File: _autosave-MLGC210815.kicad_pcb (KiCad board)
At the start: 2 copper layers, 95 x 24 mm, 110 parts, among them J1 PinHeader_01x06_Male, J2 USB-B-04PFHTW, J3 PinHeader_01x01_Male, J4 PinHeader_01x01_Male, J5 PinHeader_01x02_Male, Q1 P-MOSFET_SI2315BDS-T1-E3, Q2 NPN_BC817, Q3 NPN_BC817, Q4 P-MOSFET_SI2315BDS-T1-E3, SW1 Switch-Tact_OMRON-B3F-3100, SW2 Switch-Tact_OMRON-B3F-3100, SW3 Switch-Tact_OMRON-B3F-3100, U1 PIC32MX170F256B-ISS, U2 OPA_MCP6V36T-E_OT, U3 LDO_MCP1700T-3302E_TT, U4 SENSOR_BMA250E, U5 INTERFACE_FT230XS, U6 BATTERY_MCP73833-FCI_UN, U7 DISPLAY_REX012832FWPP3N01, Y1 Crystal_SMD3225_12MHz

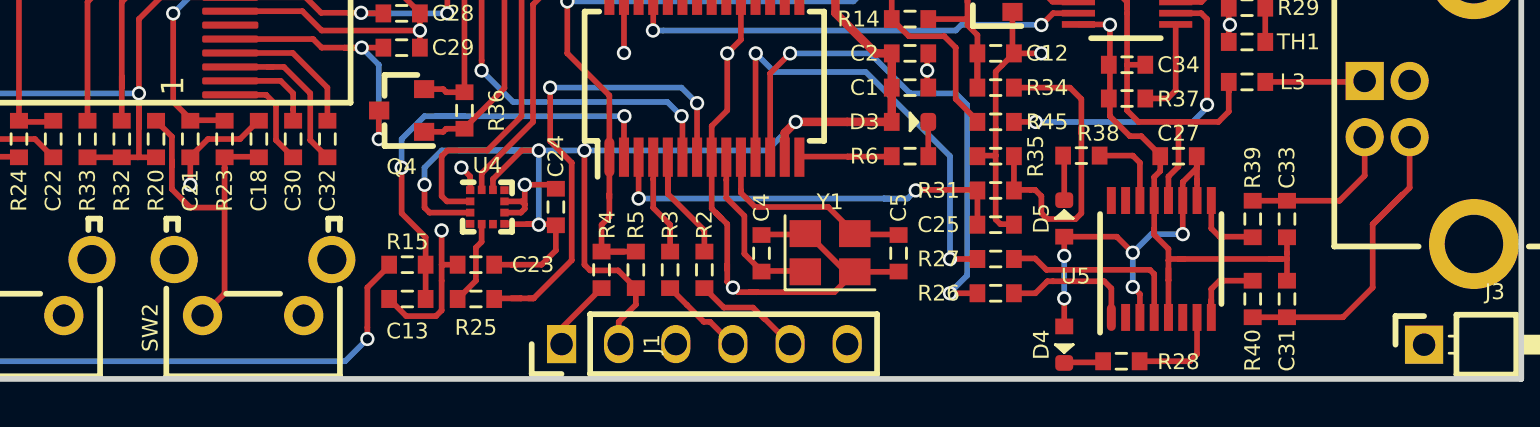
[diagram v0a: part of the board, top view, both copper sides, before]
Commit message: update
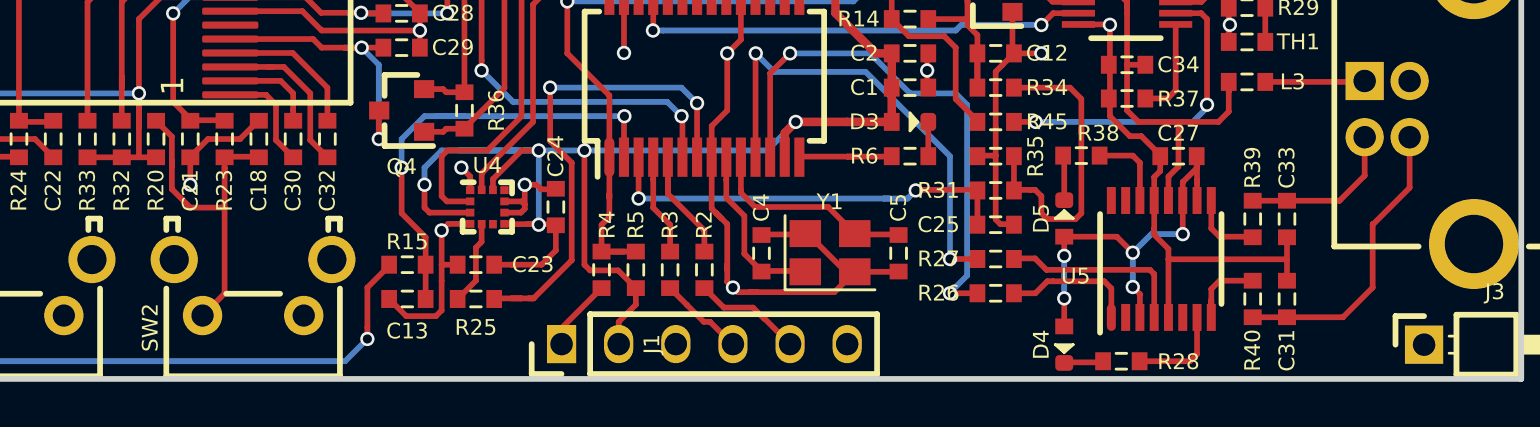
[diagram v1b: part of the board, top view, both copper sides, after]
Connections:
- U4 pad 4: Net-(U4-Pad4) -> GNDD
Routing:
- net /D+: track 15.9 -> 13.3 mm
